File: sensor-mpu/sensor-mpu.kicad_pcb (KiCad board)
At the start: 2 copper layers, 31.2 x 42 mm, 28 parts, among them J1 JST SH1.0, Q1 BSS138, Q2 BSS138, U1 LN1134A182MR-G, U2 MPU-9250, U3 MAX30102

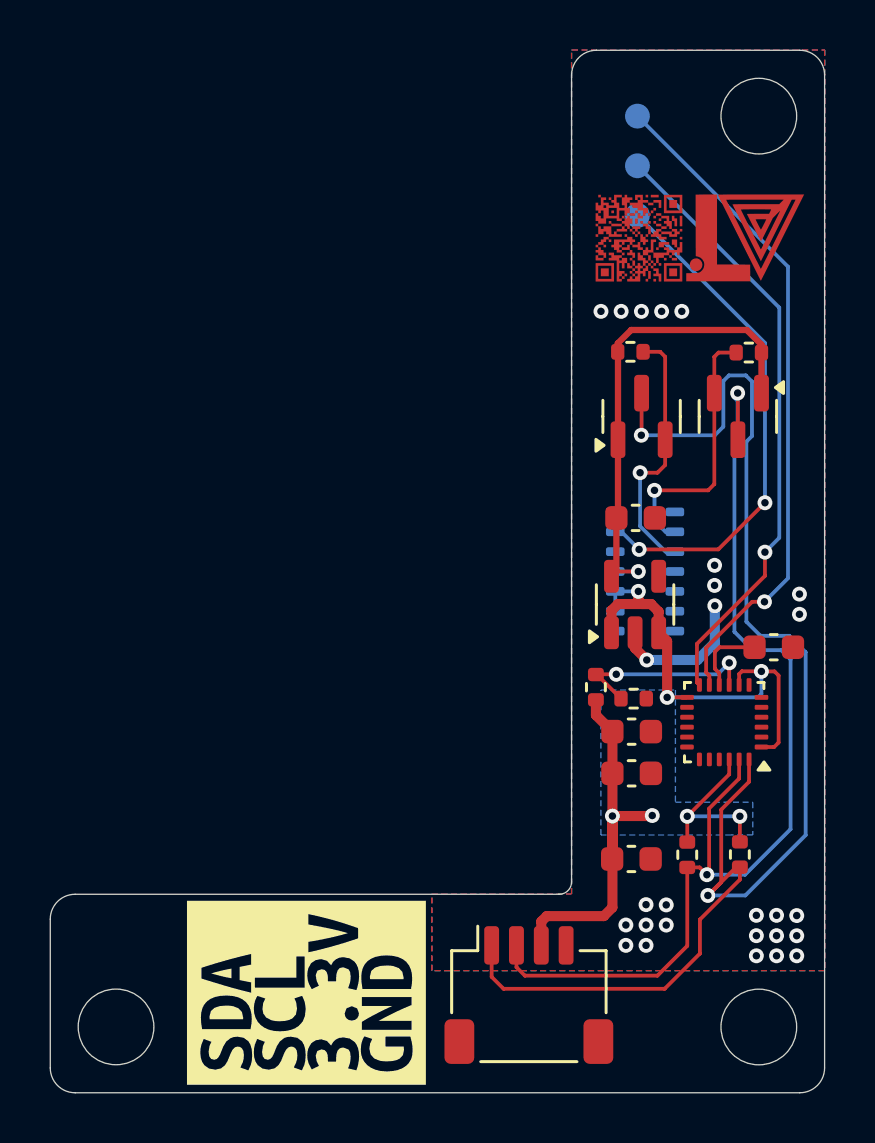
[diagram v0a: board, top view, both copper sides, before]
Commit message: panelize sensor board
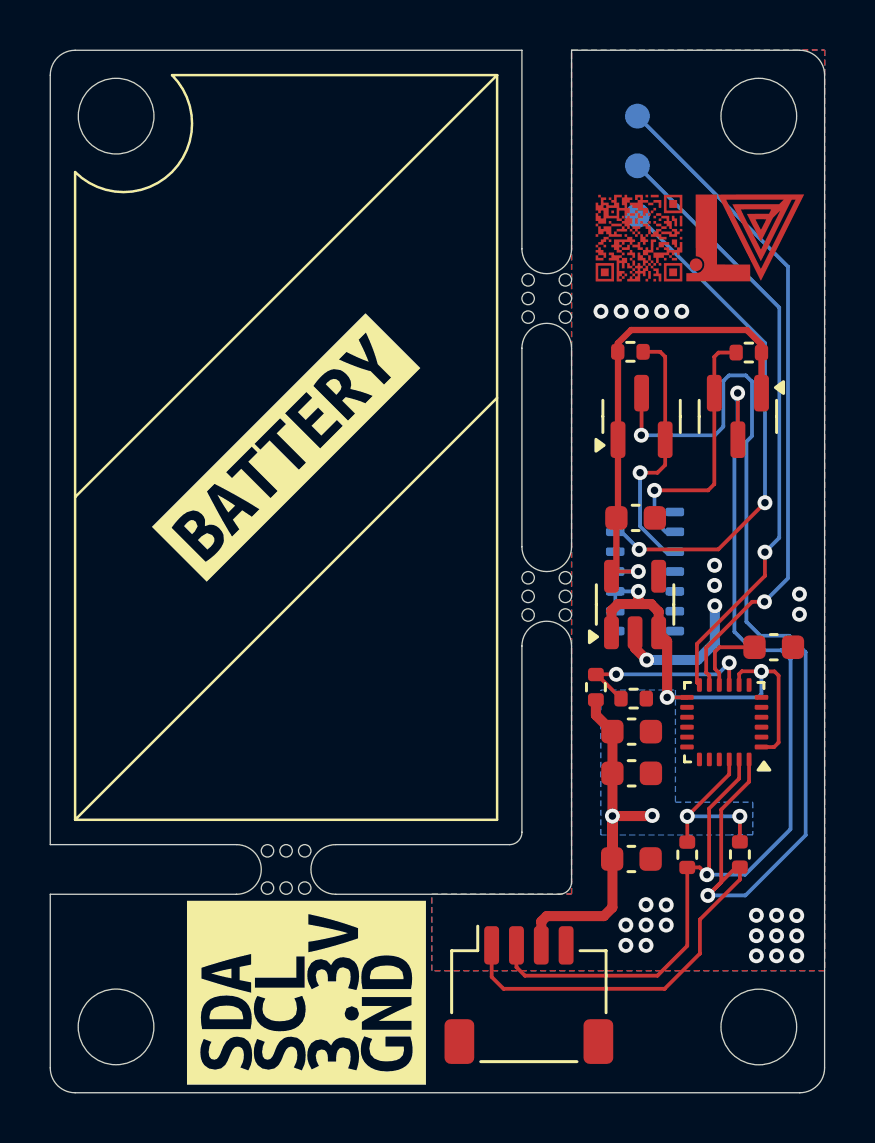
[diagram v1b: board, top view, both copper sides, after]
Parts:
- added kibuzzard-68103EF6: G***, kibuzzard-68103EF6, F.Cu at (183.0, 60.8)
- added kibuzzard-68103EF6: G***, kibuzzard-68103EF6, B.Cu at (183.0, 60.8)
- added mouse-bite-2mm-slot: VAL**, Panelization Pretty:mouse-bite-2mm-slot, F.Cu at (183.0, 77.8)
- added mouse-bite-2mm-slot: VAL**, Panelization Pretty:mouse-bite-2mm-slot, F.Cu at (193.5, 66.8)
- added mouse-bite-2mm-slot: VAL**, Panelization Pretty:mouse-bite-2mm-slot, F.Cu at (193.5, 54.8)
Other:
- outline, holes or cut-outs redrawn
